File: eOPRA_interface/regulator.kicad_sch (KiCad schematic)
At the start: 10 parts, among them U14 AP2205-50, U34 AP2213-8_SOIC

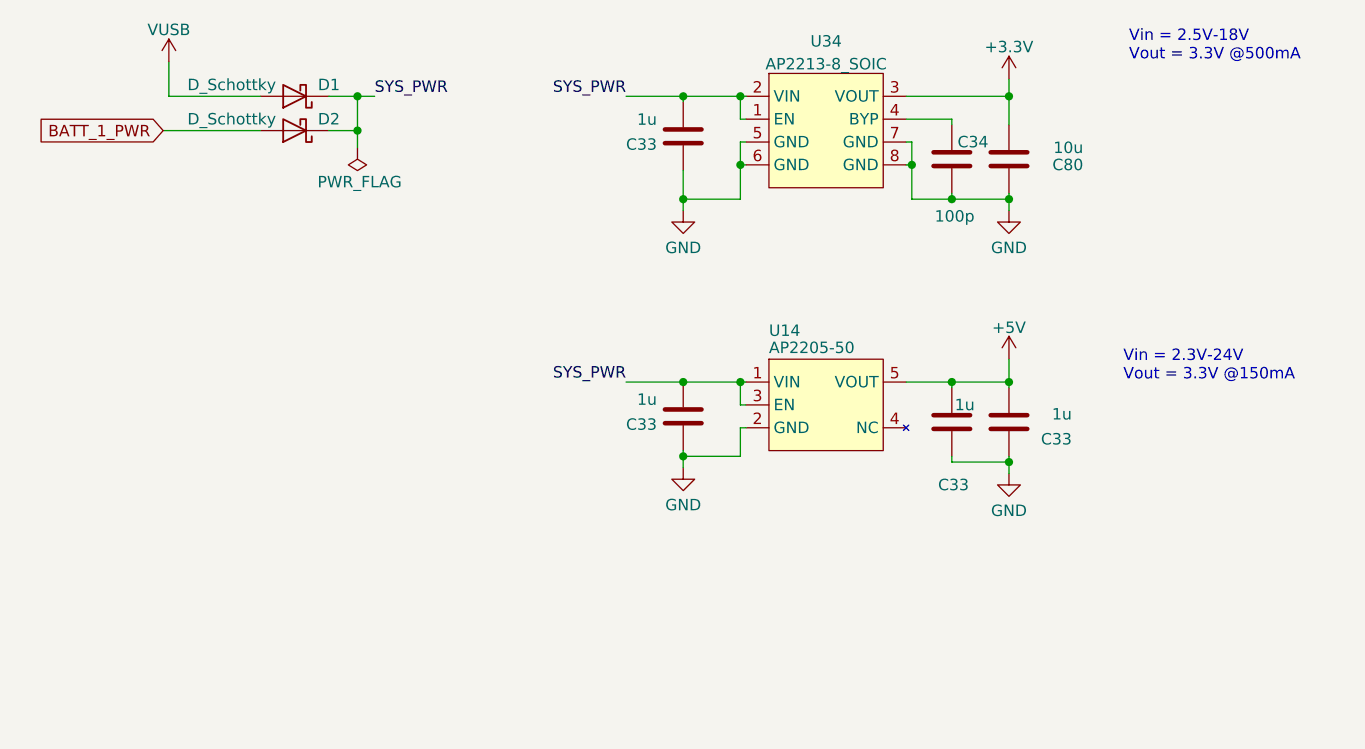
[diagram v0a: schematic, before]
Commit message: schematic v1.0 finished
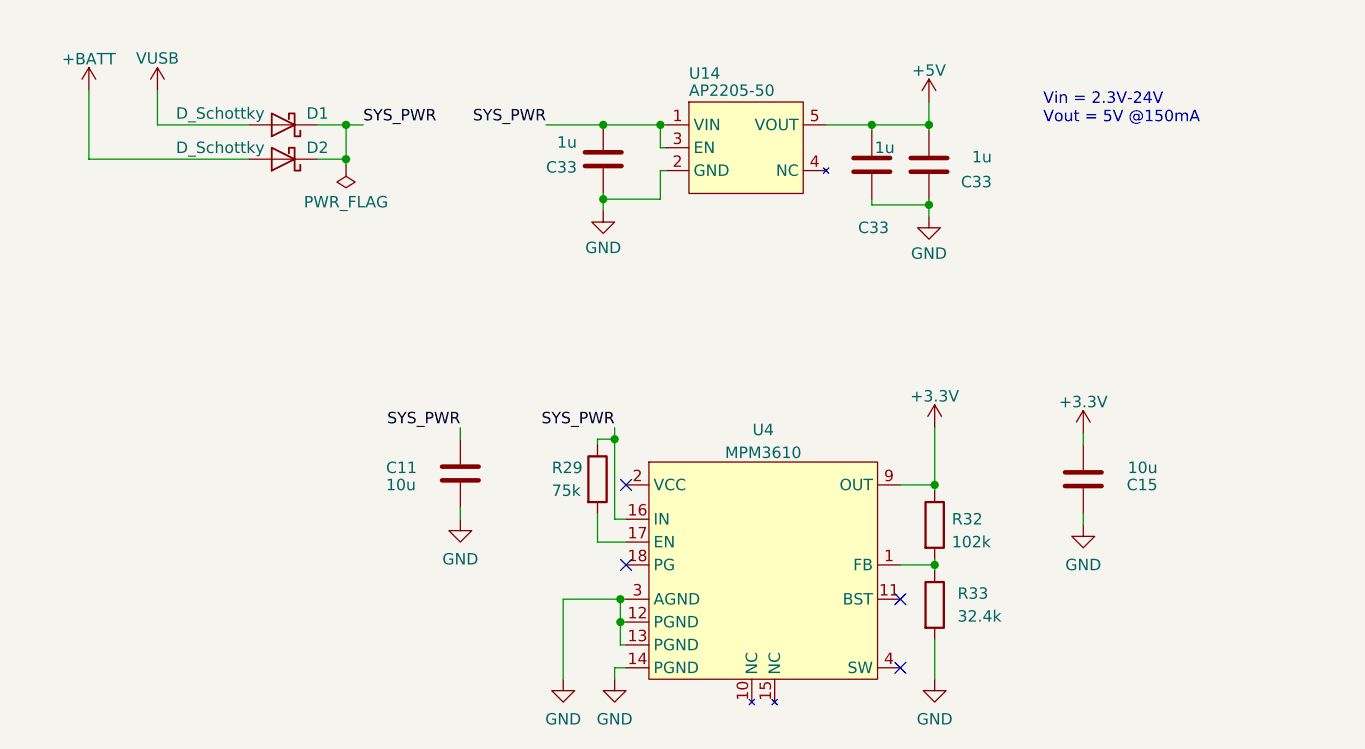
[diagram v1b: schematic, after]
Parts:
- removed C33: 1u, 2_Passives_Capacitors_SMD_IPC:C_1608_603_B, symbol 2.passive:C
- removed C34: 100p, 2_Passives_Capacitors_SMD_IPC:C_1608_603_B, symbol 2.passive:C
- removed C80: 10u, 2_Passives_Capacitors_SMD_IPC:C_2012_805_B, symbol 2.passive:C
- removed U34: AP2213-8_SOIC, 1_Semi_Misc:SOIC-8_3.9x4.9mm_P1.27mm, symbol 1.semi.ic.pmic.voltagereg:AP2213-8_SOIC
- added C11, C15: 10u, 2_Passives_Capacitors_SMD_IPC:C_2012_805_B, symbol 2.passive:C
- added R29: 75k, 2_Passives_Resistors_SMD_IPC:R_1608_603_B, symbol 2.passive:R
- added R32: 102k, 2_Passives_Resistors_SMD_IPC:R_1608_603_B, symbol 2.passive:R
- added R33: 32.4k, 2_Passives_Resistors_SMD_IPC:R_1608_603_B, symbol 2.passive:R
- added U4: MPM3610, 1_Semi_QFN:20-PowerLQFN, symbol 1.semi.ic.pmic.voltagereg:MPM3610
- D1, D2: PN TBD -> (none)
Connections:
- net +3V3: now also C15.2, R32.1, U4.9 (OUT)
- net GND: now also C11.2, C15.1, R33.2, U4.12 (PGND), U4.13 (PGND), U4.14 (PGND), U4.3 (AGND)
- net SYS_PWR: now also C11.1, R29.1, U4.16 (IN)
- net BATT_1_PWR renamed +BATT
- new net: R32.2, R33.1, U4.1 (FB)
- new net: R29.2, U4.17 (EN)
- no-connect marks 0 -> 4
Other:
- note added: "Vin = 2.3V-24V Vout = 5V @150mA"
- note removed: "Vin = 2.3V-24V Vout = 3.3V @150mA"
- note removed: "Vin = 2.5V-18V Vout = 3.3V @500mA"
- moved on the sheet: C33, D1, D2, U14

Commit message: Version updates
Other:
- company: (none) -> Massachusetts Institute of Technology / MIT Media Lab
- title: (none) -> eOPRA Switch / Stimulation Controller
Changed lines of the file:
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@@
 (kicad_sch (version 20230121) (generator eeschema)
   (paper "A4")
+  (title_block
+    (title "eOPRA Switch / Stimulation Controller")
+    (date "2023-08-01")
+    (rev "1.0")
+    (company "Massachusetts Institute of Technology / MIT Media Lab")
+  )
   (junction (at 125.095 86.36) (diameter 0) (color 0 0 0 0)
   )
